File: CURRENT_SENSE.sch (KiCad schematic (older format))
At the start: 21 parts, among them Q2L1 MMBT5551, Q2R1 MMBT5551, U14 3PEAK TP09-SR

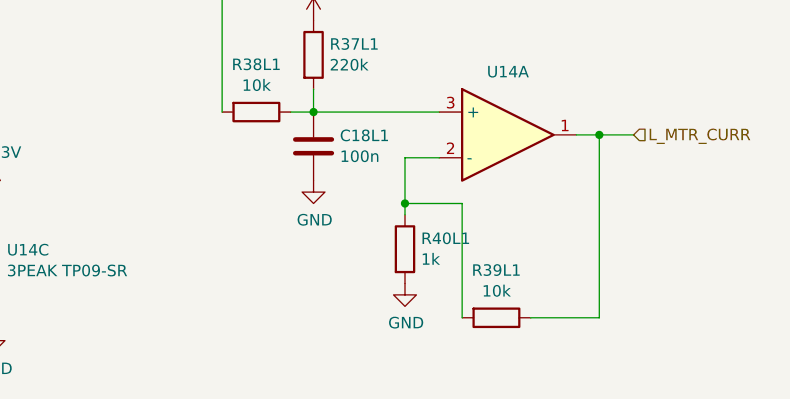
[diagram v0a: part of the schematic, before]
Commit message: fix some errors
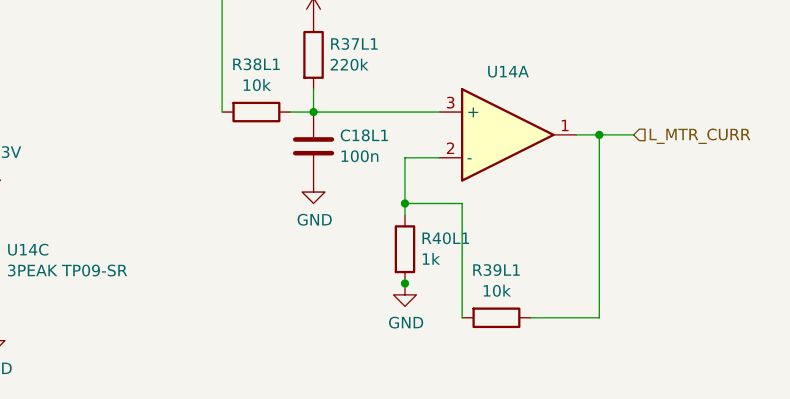
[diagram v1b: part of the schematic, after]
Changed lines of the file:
@@
 	1    0    0    -1
 $EndComp
+Connection ~ 6950 5150
 $EndSCHEMATC

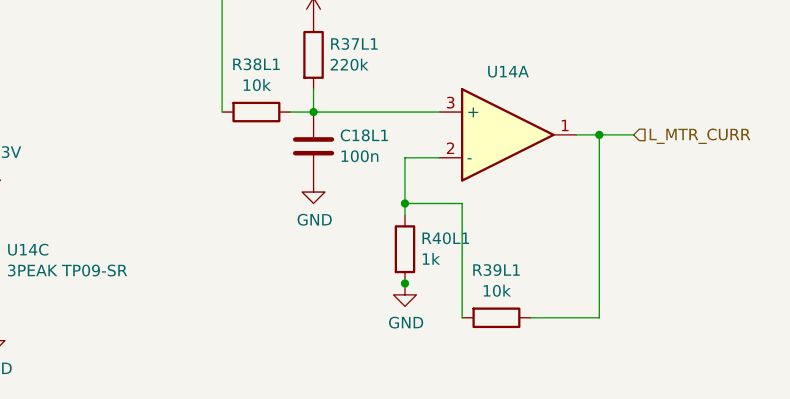
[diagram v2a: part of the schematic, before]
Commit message: Add TVS diode, fuse to 15 V supply
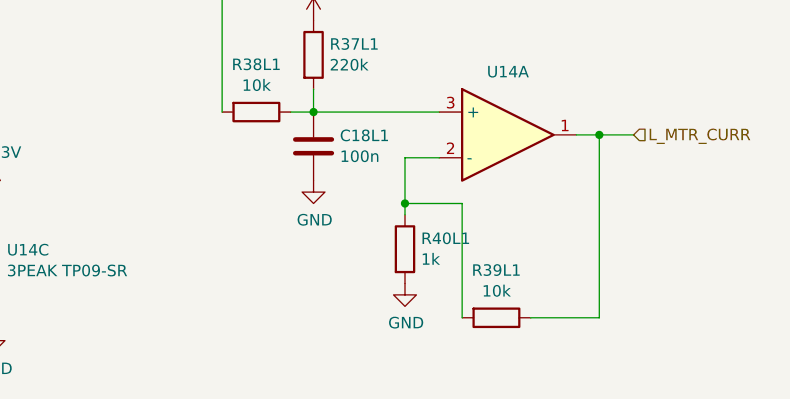
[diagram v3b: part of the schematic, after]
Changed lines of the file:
@@
 	1    0    0    -1
 $EndComp
-Connection ~ 6950 5150
 $EndSCHEMATC
